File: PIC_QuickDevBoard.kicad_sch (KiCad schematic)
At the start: 36 parts, among them J1 Conn_01x08_Pin, J10 VCC Lines, J2 Conn_01x08_Pin, J3 Conn_01x08_Pin, J4 PowerSource, J5 PICKitConnector, J6 USB_B_Micro, J7 PGEC_LINES, J8 PGED_LINES, J9 MCLR_LINES, SW1 SW_Push, U1 PIC24F, U2 PIC16F84, U3 LDA33A, U4 PIC16F1459-IP, Y1 Crystal

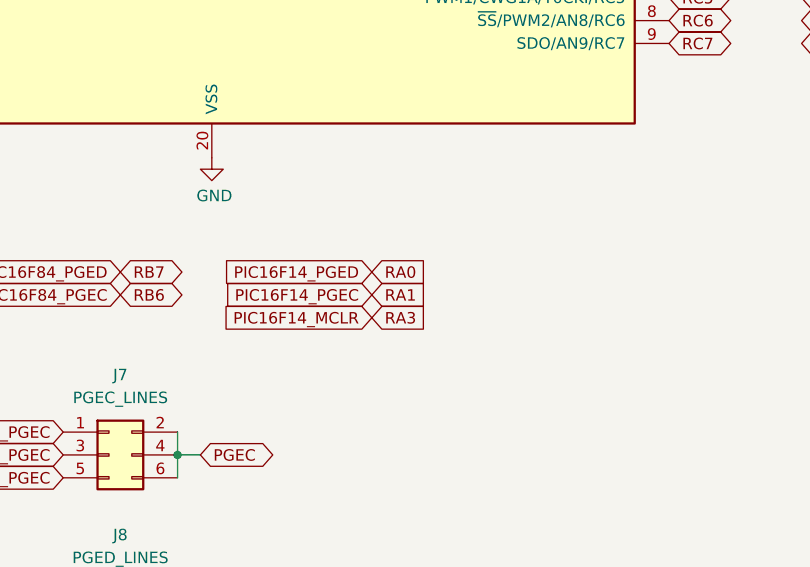
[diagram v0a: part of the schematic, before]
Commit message: Revision 2.2
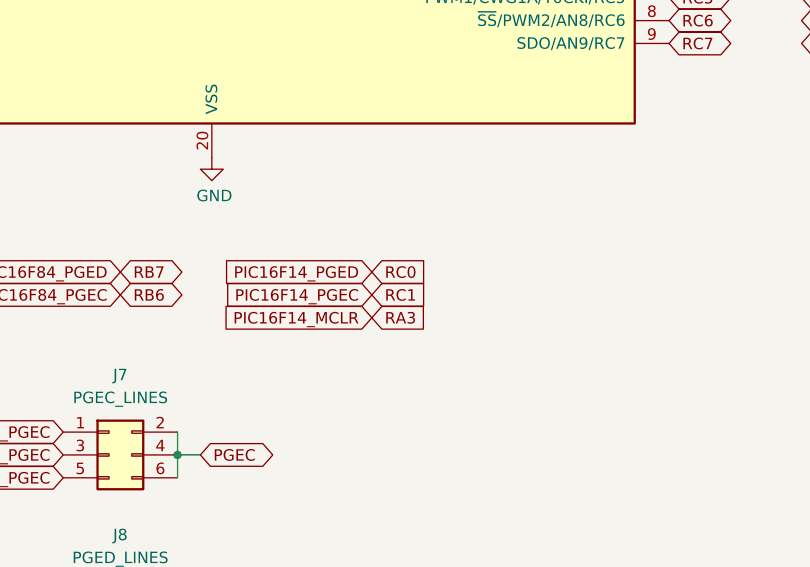
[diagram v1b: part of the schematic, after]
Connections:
- net PIC24_PGEC is gone; now on net PIC16F14_PGEC: J2.2 (Pin_2), J7.1 (Pin_1), U1.5 (RB1), U2.7 (RB1), U4.15 (ICSPCLK/~{CWGFLT}/C2IN-/C1IN-/AN5/RC1)
- net PIC24_PGED is gone; now on net PIC16F14_PGED: J2.1 (Pin_1), J8.1 (Pin_1), U1.4 (RB0), U2.6 (INT/RB0), U4.16 (ICSPDAT/C2IN+/C1IN+/Vref+/AN4/RC0)
- net PIC16F14_PGEC: no longer J1.2 (Pin_2), R4.1, U1.3 (RA1), U2.18 (RA1), U4.18 (RA1/D-/ICSPCLK)
- net PIC16F14_PGED: no longer J1.1 (Pin_1), R5.2, SW1.2, U1.2 (RA0), U2.17 (RA0), U4.19 (RA0/D+/ICSPDAT)
- new net RA0: J1.1 (Pin_1), R5.2, SW1.2, U1.2 (RA0), U2.17 (RA0), U4.19 (RA0/D+/ICSPDAT)
- new net RA1: J1.2 (Pin_2), R4.1, U1.3 (RA1), U2.18 (RA1), U4.18 (RA1/D-/ICSPCLK)
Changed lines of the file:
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@@
 	(title_block
 		(title "PIC24 & PIC16F84 Programmer & Dev Board")
-		(date "2024-04-13")
-		(rev "2.1")
+		(date "2024-05-01")
+		(rev "2.2")
 		(company "RCC 2024")
 		(comment 1 "https://github.com/costarc/PIC_QuickDevBoard")
@@
 		)
 	)
+	(global_label "RC0"
+		(shape input)
+		(at 341.63 146.05 0)
+		(fields_autoplaced yes)
+		(effects
+			(font
+				(size 1.27 1.27)
+			)
+			(justify left)
+		)
+		(property "Intersheetrefs" "${INTERSHEET_REFS}"
+			(at 348.3647 146.05 0)
+			(effects
+				(font
+					(size 1.27 1.27)
+				)
+				(justify left)
+				(hide yes)
+			)
+		)
+	)
 	(global_label "RB5"
 		(shape bidirectional)
@@
 		)
 	)
+	(global_label "RC1"
+		(shape input)
+		(at 341.63 148.59 0)
+		(fields_autoplaced yes)
+		(effects
+			(font
+				(size 1.27 1.27)
+			)
+			(justify left)
+		)
+		(property "Intersheetrefs" "${INTERSHEET_REFS}"
+			(at 348.3647 148.59 0)
+			(effects
+				(font
+					(size 1.27 1.27)
+				)
+				(justify left)
+				(hide yes)
+			)
+		)
+	)
 	(global_label "PIC16F84_MCLR"
 		(shape input)
@@
 		)
 	)
-	(global_label "RA0"
-		(shape input)
-		(at 341.63 146.05 0)
-		(fields_autoplaced yes)
-		(effects
-			(font
-				(size 1.27 1.27)
-			)
-			(justify left)
-		)
-		(property "Intersheetrefs" "${INTERSHEET_REFS}"
-			(at 348.1833 146.05 0)
-			(effects
-				(font
-					(size 1.27 1.27)
-				)
-				(justify left)
-				(hide yes)
-			)
-		)
-	)
 	(global_label "RC0"
 		(shape bidirectional)
@@
 			(effects
 				(font
-					(size 1.27 1.27)
-				)
-				(justify left)
-				(hide yes)
-			)
-		)
-	)
-	(global_label "RA1"
-		(shape input)
-		(at 341.63 148.59 0)
-		(fields_autoplaced yes)
-		(effects
-			(font
-				(size 1.27 1.27)
-			)
-			(justify left)
-		)
-		(property "Intersheetrefs" "${INTERSHEET_REFS}"
-			(at 348.1833 148.59 0)
-			(effects
-				(font
